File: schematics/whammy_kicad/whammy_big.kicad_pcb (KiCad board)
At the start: 2 copper layers, 49 parts, among them Q1 2SK2013, Q2 2SJ313, Q3 2SK2013, Q4 2SJ313, U1 OPA1637, U4 4N35, U5 4N35

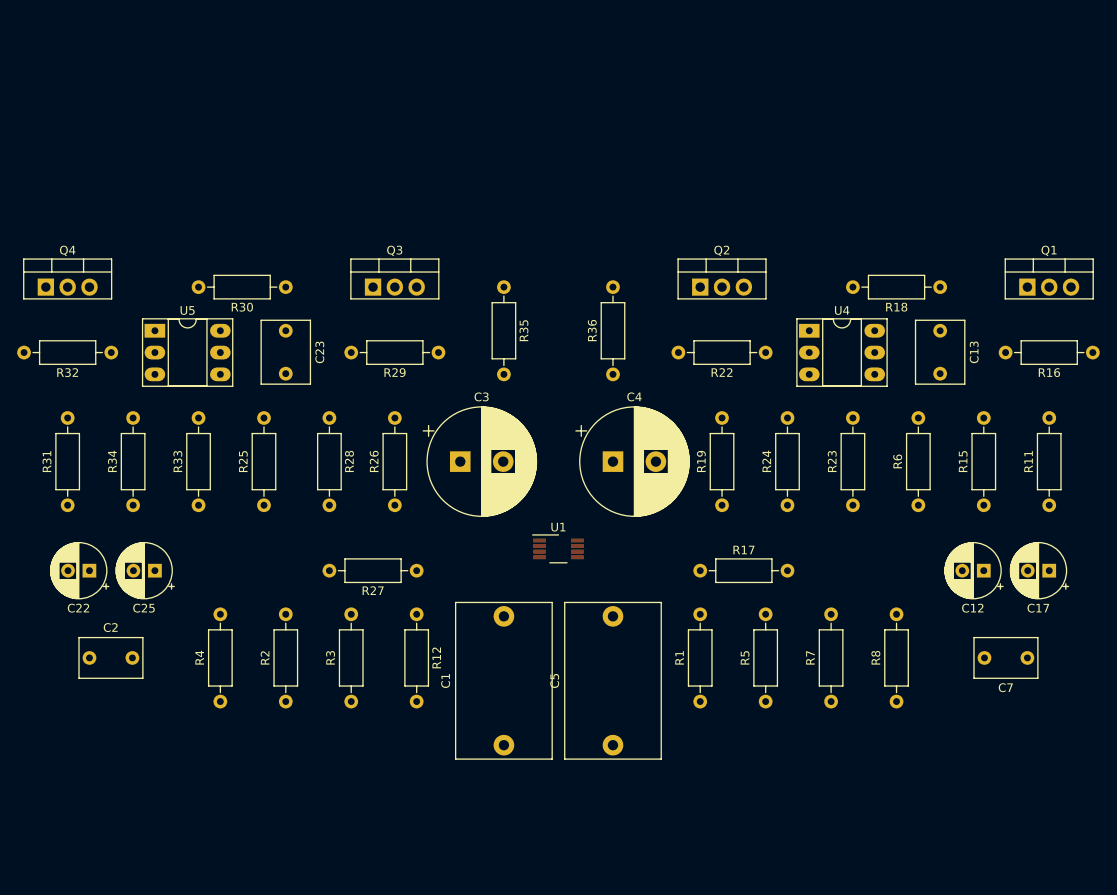
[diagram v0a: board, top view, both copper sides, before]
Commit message: Final version
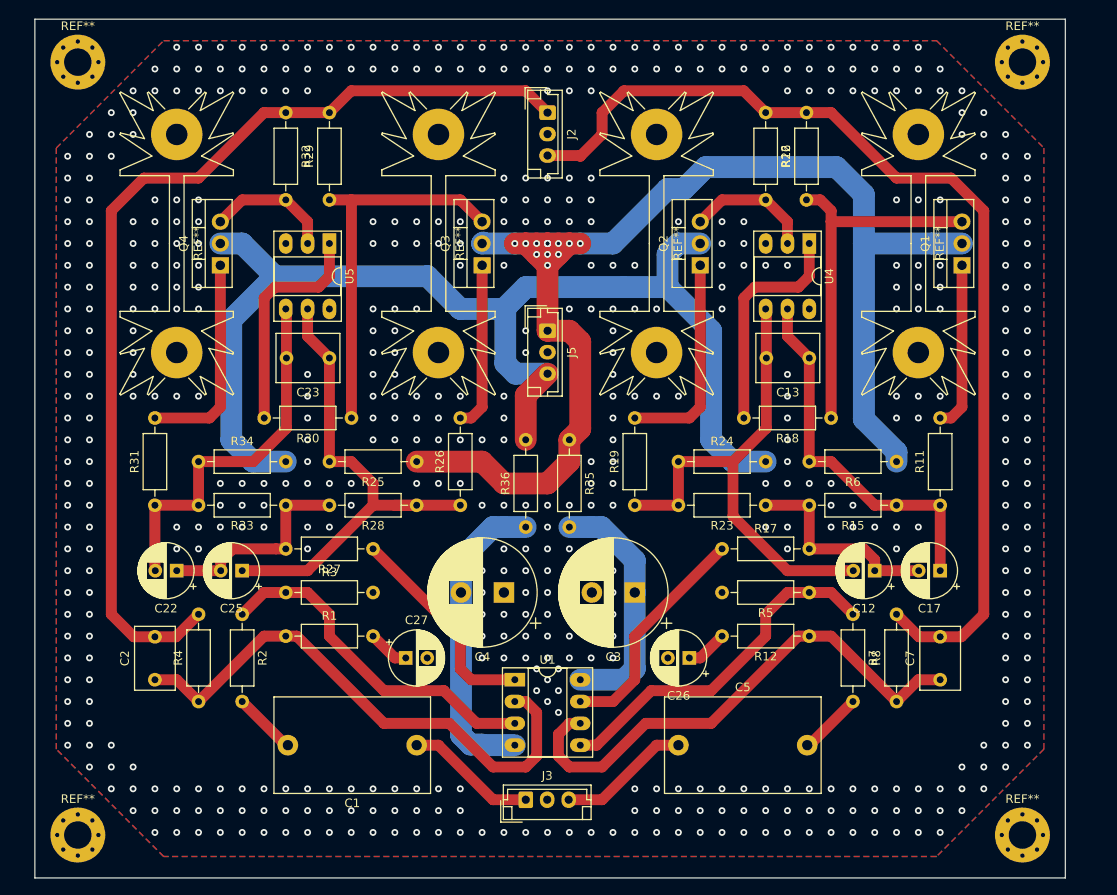
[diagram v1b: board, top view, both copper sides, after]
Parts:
- added C26: 22uF/25V, Capacitor_THT:CP_Radial_D6.3mm_P2.50mm, F.Cu at (156.2, 119.4)
- added C27: 22uF/25V, Capacitor_THT:CP_Radial_D6.3mm_P2.50mm, F.Cu at (123.2, 119.4)
- added J2: Conn_01x03, Connector_JST:JST_EH_B3B-EH-A_1x03_P2.50mm_Vertical, F.Cu at (139.7, 55.9)
- added J3: Conn_01x03, Connector_JST:JST_EH_B3B-EH-A_1x03_P2.50mm_Vertical, F.Cu at (137.2, 135.9)
- added J5: Conn_01x03, Connector_JST:JST_EH_B3B-EH-A_1x03_P2.50mm_Vertical, F.Cu at (139.7, 81.3)
- added REF**: MountingHole_3.2mm_M3_Pad_Via, MountingHole:MountingHole_3.2mm_M3_Pad_Via, F.Cu at (195.0, 140.0)
- added REF**: MountingHole_3.2mm_M3_Pad_Via, MountingHole:MountingHole_3.2mm_M3_Pad_Via, F.Cu at (85.0, 140.0)
- added REF**: MountingHole_3.2mm_M3_Pad_Via, MountingHole:MountingHole_3.2mm_M3_Pad_Via, F.Cu at (195.0, 50.0)
- added REF**: MountingHole_3.2mm_M3_Pad_Via, MountingHole:MountingHole_3.2mm_M3_Pad_Via, F.Cu at (85.0, 50.0)
- added REF**: Heatsink_Fischer_SK104-STC-STIC_35x13mm_2xDrill2.5mm, Heatsink:Heatsink_Fischer_SK104-STC-STIC_35x13mm_2xDrill2.5mm, F.Cu at (182.9, 71.1)
- added REF**: Heatsink_Fischer_SK104-STC-STIC_35x13mm_2xDrill2.5mm, Heatsink:Heatsink_Fischer_SK104-STC-STIC_35x13mm_2xDrill2.5mm, F.Cu at (152.4, 71.1)
- added REF**: Heatsink_Fischer_SK104-STC-STIC_35x13mm_2xDrill2.5mm, Heatsink:Heatsink_Fischer_SK104-STC-STIC_35x13mm_2xDrill2.5mm, F.Cu at (127.0, 71.1)
- added REF**: Heatsink_Fischer_SK104-STC-STIC_35x13mm_2xDrill2.5mm, Heatsink:Heatsink_Fischer_SK104-STC-STIC_35x13mm_2xDrill2.5mm, F.Cu at (96.5, 71.1)
- R1, R12: value 49 -> 1K
- U1: value OPA1637 -> OPA2604; footprint Package_SO:VSSOP-8_3.0x3.0mm_P0.65mm -> Package_DIP:DIP-8_W7.62mm_Socket_LongPads
- moved R1 48.9 mm to (109.2, 116.8), turned to 0 degrees
- moved R12 45.8 mm to (170.2, 116.8), turned to 180 degrees
- moved R16 37.8 mm to (169.8, 66.0), turned to 90 degrees
- moved R32 34.5 mm to (109.2, 55.9), turned to 270 degrees
- moved R22 27.9 mm to (165.1, 55.9), turned to 270 degrees
- moved C3 25.4 mm to (149.9, 111.8), turned to 180 degrees
- moved U5 22.7 mm to (114.3, 71.1), turned to 270 degrees
- moved R29 21.8 mm to (114.3, 66.0), turned to 90 degrees
- moved R36 20.5 mm to (137.2, 104.1)
- moved Q4 20.5 mm to (101.6, 73.7), turned to 90 degrees
- moved C4 19.8 mm to (134.6, 111.8), turned to 180 degrees
- moved R18 19.8 mm to (172.7, 91.4)
- moved R35 19.3 mm to (142.2, 94.0)
- moved R25 18.5 mm to (124.5, 96.5), turned to 180 degrees
- moved R30 17.1 mm to (116.9, 91.4)
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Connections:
- net OUT+ renamed LEFT_OUT
- net OUT- renamed RIGHT_OUT
- R1 pad 1: Net-(C7-Pad1) -> Net-(C2-Pad1)
- R1 pad 2: Net-(R1-Pad2) -> Net-(C27-Pad1)
- R12 pad 1: Net-(R12-Pad1) -> Net-(C7-Pad1)
- R12 pad 2: Net-(C2-Pad1) -> Net-(C26-Pad1)
- R2 pad 1: Net-(C2-Pad1) -> Net-(R2-Pad1)
- R3 pad 1: Net-(C2-Pad1) -> Net-(R2-Pad1)
- R5 pad 1: Net-(C7-Pad1) -> Net-(R5-Pad1)
- R7 pad 1: Net-(C7-Pad1) -> Net-(R5-Pad1)
- U1 pad 1: Net-(R12-Pad1) -> Net-(R27-Pad1)
- U1 pad 2: GND -> Net-(C2-Pad1)
- U1 pad 3: Net-(C3-Pad1) -> Net-(R2-Pad1)
- U1 pad 4: Net-(R27-Pad1) -> Net-(C4-Pad2)
- U1 pad 5: Net-(R17-Pad1) -> Net-(R5-Pad1)
- U1 pad 6: Net-(C4-Pad2) -> Net-(C7-Pad1)
- U1 pad 7: GND -> Net-(R17-Pad1)
- U1 pad 8: Net-(R1-Pad2) -> Net-(C3-Pad1)
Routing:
- net +15V: track 0.00 -> 164.4 mm, vias 0 -> 13
- net -15V: track 0.00 -> 140.8 mm
- net LEFT_OUT: track 0.00 -> 120.6 mm, vias 0 -> 1
- net RIGHT_OUT: track 0.00 -> 117.1 mm
- net Net-(C2-Pad1): track 0.00 -> 63.6 mm
- net Net-(C7-Pad1): track 0.00 -> 61.1 mm
- net Net-(C12-Pad2): track 0.00 -> 58.9 mm
- net Net-(C23-Pad1): track 0.00 -> 58.6 mm
- net Net-(Q3-Pad3): track 0.00 -> 44.2 mm
- net Net-(C13-Pad1): track 0.00 -> 43.8 mm
- net Net-(C22-Pad2): track 0.00 -> 43.6 mm
- net Net-(Q1-Pad3): track 0.00 -> 42.8 mm
- net Net-(R5-Pad1): track 0.00 -> 41.7 mm
- net Net-(R2-Pad1): track 0.00 -> 40.6 mm
- net Net-(C4-Pad2): track 0.00 -> 36.3 mm
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- added copper zone on B.Cu, net GND
- added copper zone on F.Cu, net GND
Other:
- board outline added: 120 x 100 mm
